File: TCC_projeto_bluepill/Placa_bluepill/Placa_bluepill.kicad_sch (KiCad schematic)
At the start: 40 parts

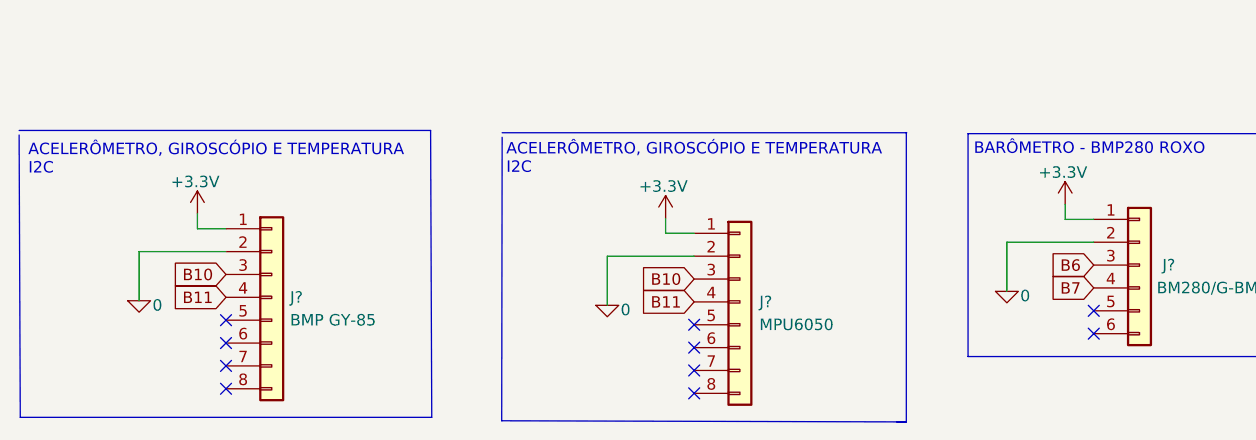
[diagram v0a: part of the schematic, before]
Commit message: mod
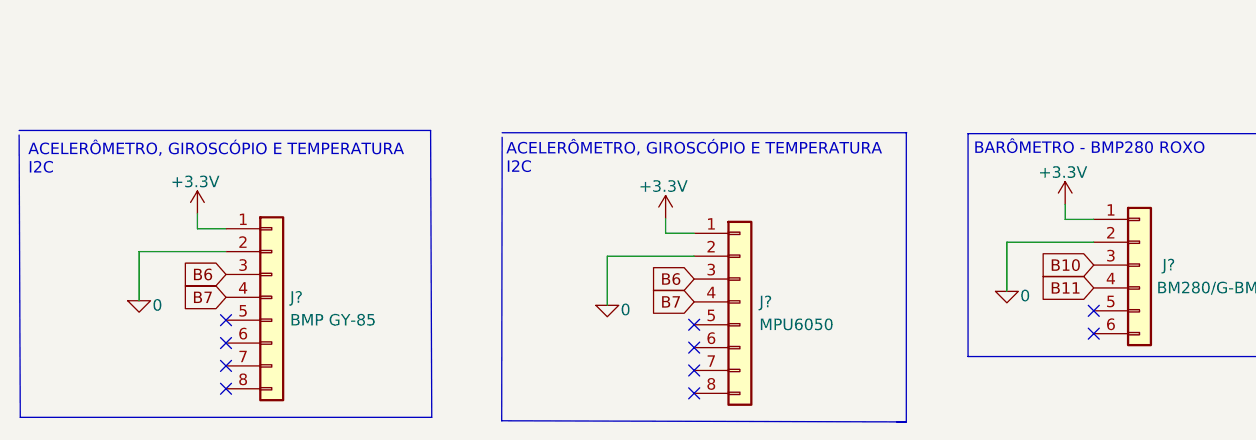
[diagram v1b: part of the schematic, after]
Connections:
- net B10: now also J?.3 (Pin_3); no longer J?.3 (Pin_3), J?.3 (Pin_3)
- net B11: now also J?.4 (Pin_4); no longer J?.4 (Pin_4), J?.4 (Pin_4)
- net B6: now also J?.3 (Pin_3), J?.3 (Pin_3); no longer J?.3 (Pin_3)
- net B7: now also J?.4 (Pin_4), J?.4 (Pin_4); no longer J?.4 (Pin_4)
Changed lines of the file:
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@@
-    )
-  )
-  (global_label "B7" (shape input) (at 135.8392 179.1208 180) (fields_autoplaced)
-    (effects (font (size 1.27 1.27)) (justify right))
-    (property "Intersheet References" "${INTERSHEET_REFS}" (id 0) (at 130.9466 179.0414 0)
-      (effects (font (size 1.27 1.27)) (justify right) hide)
     )
   )
@@
     )
   )
-  (global_label "B11" (shape input) (at 39.4208 180.1622 180) (fields_autoplaced)
-    (effects (font (size 1.27 1.27)) (justify right))
-    (property "Intersheet References" "${INTERSHEET_REFS}" (id 0) (at 33.3187 180.0828 0)
+  (global_label "B6" (shape input) (at 91.44 178.1302 180) (fields_autoplaced)
+    (effects (font (size 1.27 1.27)) (justify right))
+    (property "Intersheet References" "${INTERSHEET_REFS}" (id 0) (at 86.5474 178.0508 0)
+      (effects (font (size 1.27 1.27)) (justify right) hide)
+    )
+  )
+  (global_label "B6" (shape input) (at 39.4208 177.6222 180) (fields_autoplaced)
+    (effects (font (size 1.27 1.27)) (justify right))
+    (property "Intersheet References" "${INTERSHEET_REFS}" (id 0) (at 34.5282 177.5428 0)
       (effects (font (size 1.27 1.27)) (justify right) hide)
     )
@@
     )
   )
+  (global_label "B10" (shape input) (at 135.8392 176.5808 180) (fields_autoplaced)
+    (effects (font (size 1.27 1.27)) (justify right))
+    (property "Intersheet References" "${INTERSHEET_REFS}" (id 0) (at 129.7371 176.5014 0)
+      (effects (font (size 1.27 1.27)) (justify right) hide)
+    )
+  )
+  (global_label "B7" (shape input) (at 91.44 180.6702 180) (fields_autoplaced)
+    (effects (font (size 1.27 1.27)) (justify right))
+    (property "Intersheet References" "${INTERSHEET_REFS}" (id 0) (at 86.5474 180.5908 0)
+      (effects (font (size 1.27 1.27)) (justify right) hide)
+    )
+  )
   (global_label "Pin_BUZZER" (shape input) (at 236.3724 78.9432 180) (fields_autoplaced)
     (effects (font (size 1.27 1.27)) (justify right))
@@
     )
   )
+  (global_label "B7" (shape input) (at 39.4208 180.1622 180) (fields_autoplaced)
+    (effects (font (size 1.27 1.27)) (justify right))
+    (property "Intersheet References" "${INTERSHEET_REFS}" (id 0) (at 34.5282 180.0828 0)
+      (effects (font (size 1.27 1.27)) (justify right) hide)
+    )
+  )
   (global_label "OUT1" (shape input) (at 23.495 92.075 180) (fields_autoplaced)
     (effects (font (size 1.27 1.27)) (justify right))
@@
     )
   )
-  (global_label "B10" (shape input) (at 39.4208 177.6222 180) (fields_autoplaced)
-    (effects (font (size 1.27 1.27)) (justify right))
-    (property "Intersheet References" "${INTERSHEET_REFS}" (id 0) (at 33.3187 177.5428 0)
+  (global_label "B11" (shape input) (at 135.8392 179.1208 180) (fields_autoplaced)
+    (effects (font (size 1.27 1.27)) (justify right))
+    (property "Intersheet References" "${INTERSHEET_REFS}" (id 0) (at 129.7371 179.0414 0)
       (effects (font (size 1.27 1.27)) (justify right) hide)
     )
@@
     (property "Intersheet References" "${INTERSHEET_REFS}" (id 0) (at 250.1006 116.151 0)
       (effects (font (size 1.27 1.27)) (justify left) hide)
-    )
-  )
-  (global_label "B10" (shape input) (at 91.44 178.1302 180) (fields_autoplaced)
-    (effects (font (size 1.27 1.27)) (justify right))
-    (property "Intersheet References" "${INTERSHEET_REFS}" (id 0) (at 85.3379 178.0508 0)
-      (effects (font (size 1.27 1.27)) (justify right) hide)
     )
   )
@@
     )
   )
-  (global_label "B6" (shape input) (at 135.8392 176.5808 180) (fields_autoplaced)
-    (effects (font (size 1.27 1.27)) (justify right))
-    (property "Intersheet References" "${INTERSHEET_REFS}" (id 0) (at 130.9466 176.5014 0)
-      (effects (font (size 1.27 1.27)) (justify right) hide)
-    )
-  )
   (global_label "A7" (shape input) (at 174.244 78.74 0) (fields_autoplaced)
     (effects (font (size 1.27 1.27)) (justify left))
@@
     )
   )
-  (global_label "B11" (shape input) (at 91.44 180.6702 180) (fields_autoplaced)
-    (effects (font (size 1.27 1.27)) (justify right))
-    (property "Intersheet References" "${INTERSHEET_REFS}" (id 0) (at 85.3379 180.5908 0)
-      (effects (font (size 1.27 1.27)) (justify right) hide)
-    )
-  )
